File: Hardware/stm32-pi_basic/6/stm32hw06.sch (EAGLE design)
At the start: 51 parts

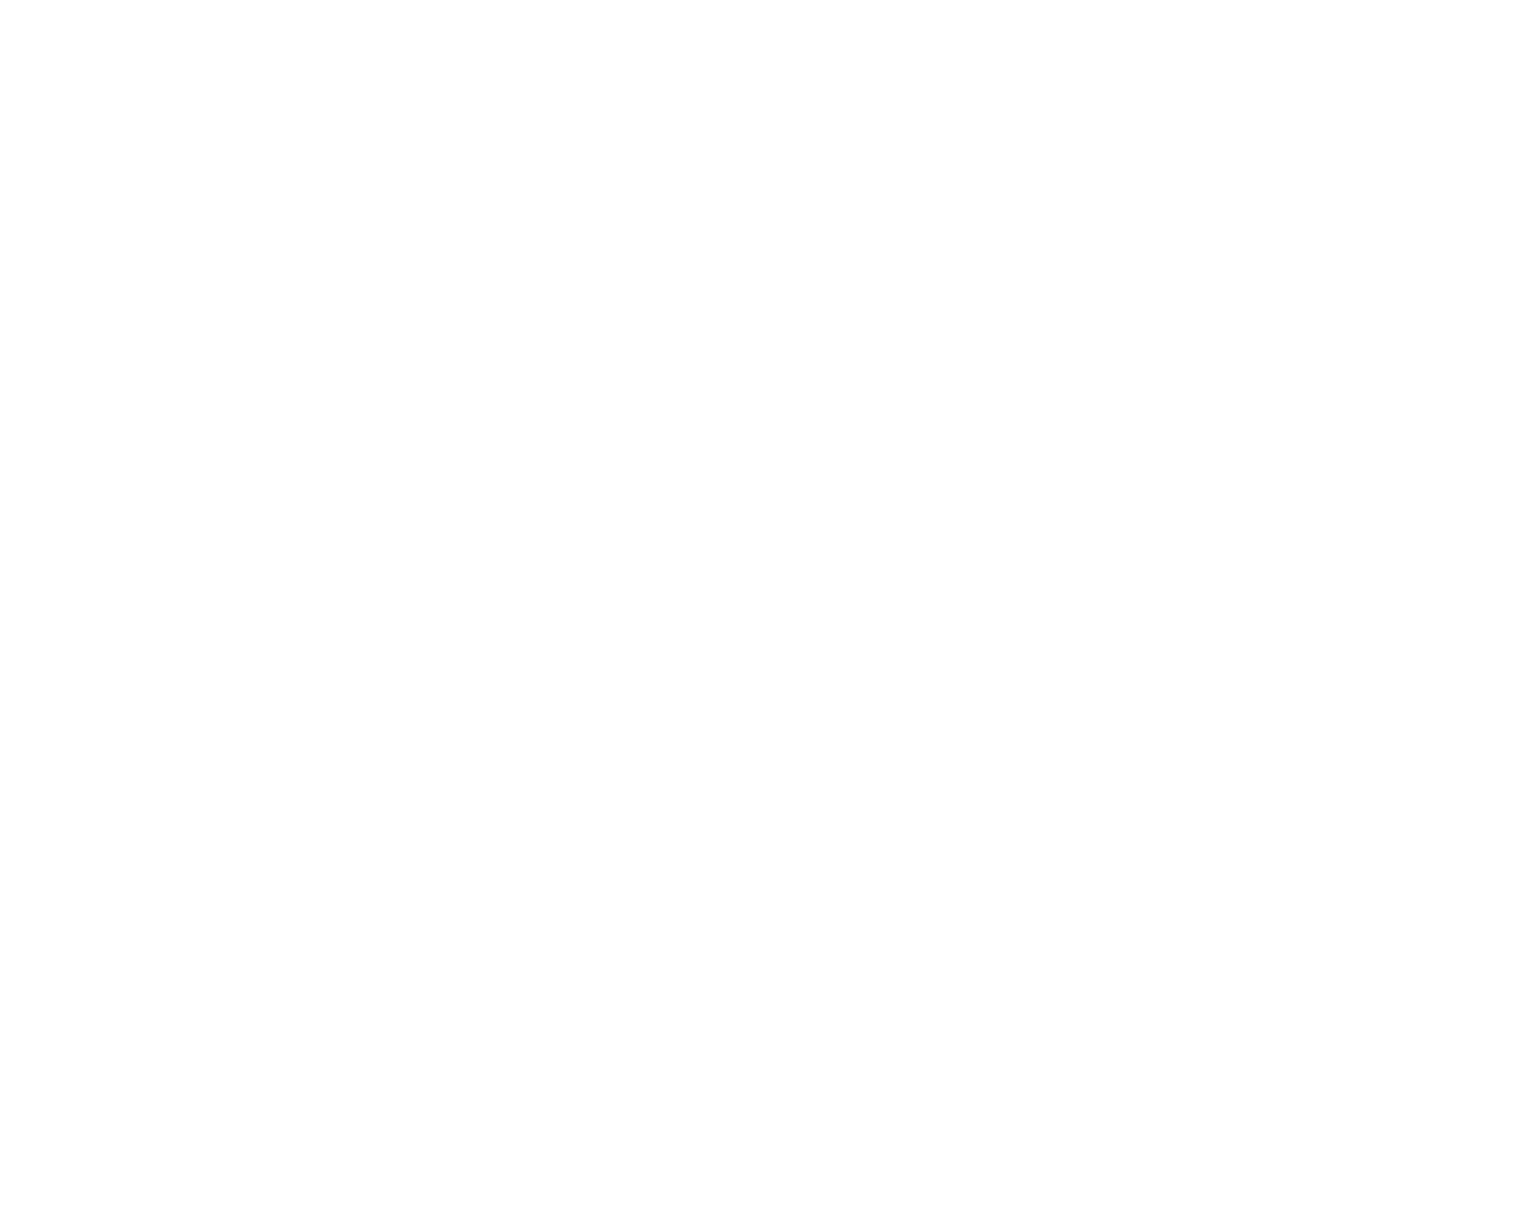
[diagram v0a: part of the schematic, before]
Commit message: deleted:    Hardware/stm32-pi_basic/6/dxfimp.scr 	modified:   Hardware/stm32-pi_basic/6/stm32hw06.brd 	modified:   Hardware/stm32-pi_basic/6/stm32hw06.sch
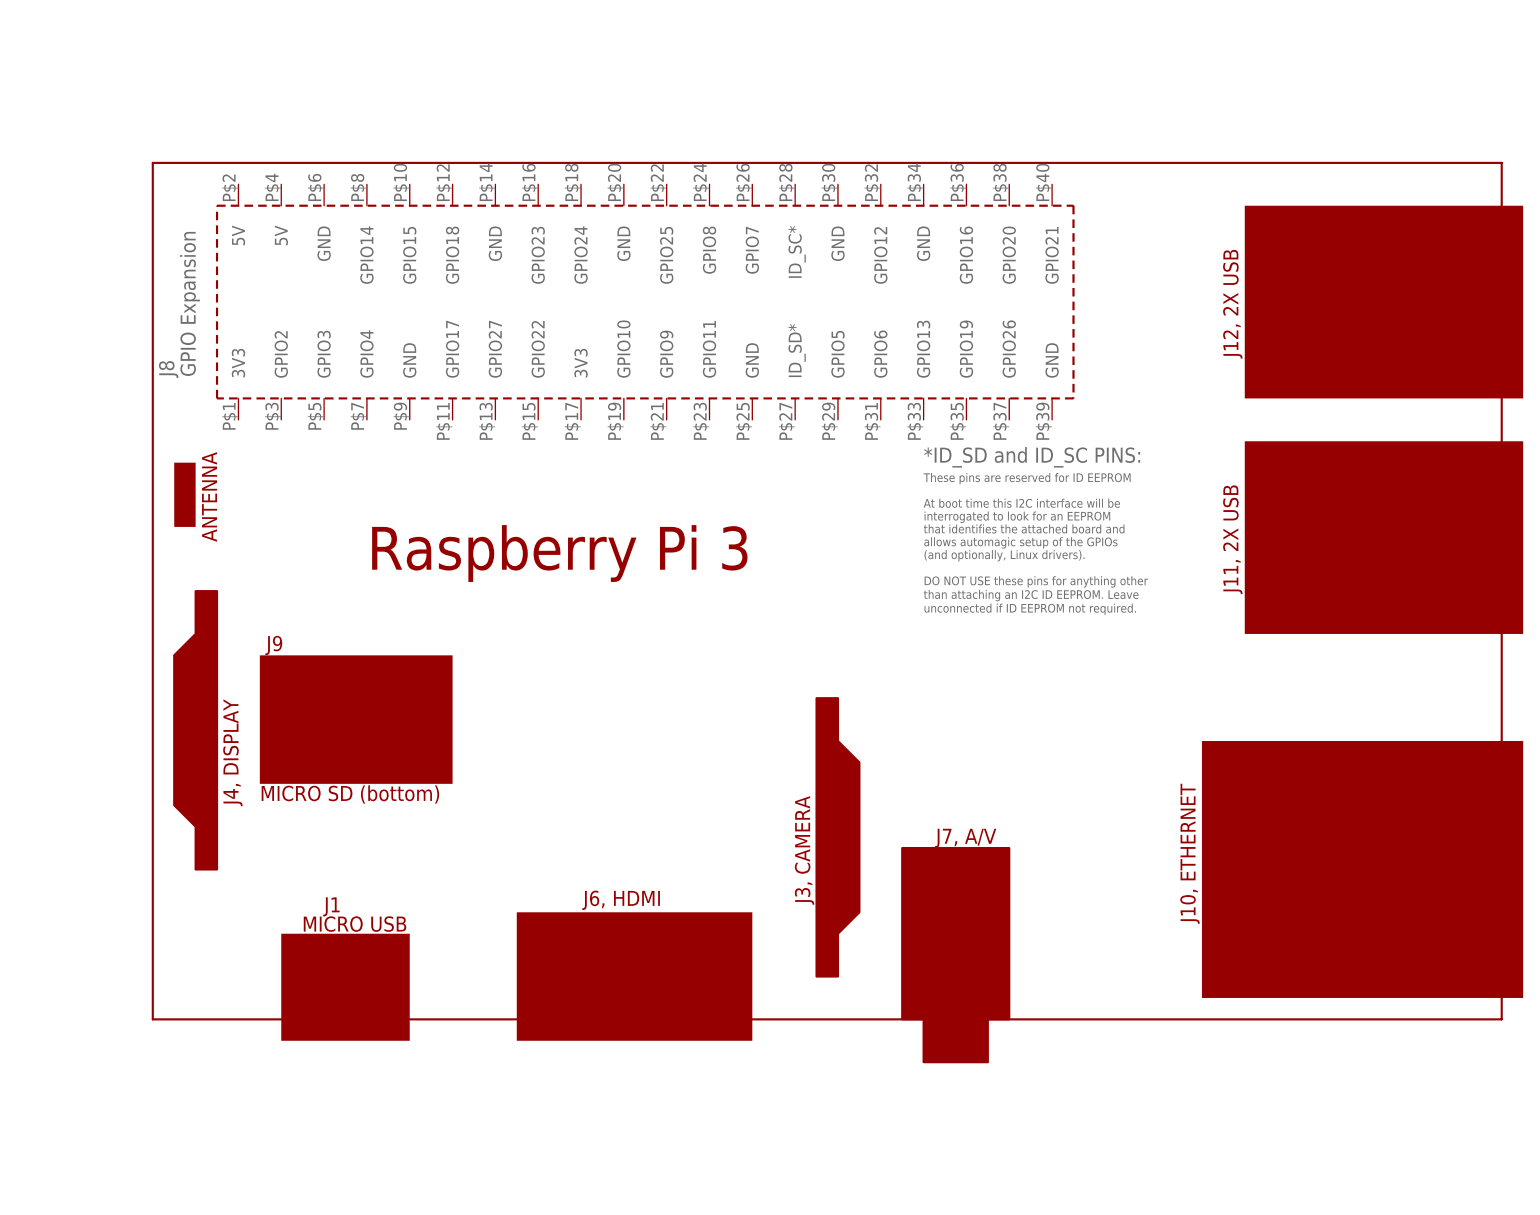
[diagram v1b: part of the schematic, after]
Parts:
- added PCB1: RPI3RPI3, e14_Rpi3_RevA+mirror-pcb:RPI3RPI3
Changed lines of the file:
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@@
 <drawing>
 <settings>
-<setting alwaysvectorfont="yes"/>
+<setting alwaysvectorfont="no"/>
 <setting keepoldvectorfont="yes"/>
 <setting verticaltext="up"/>
@@
 <part name="C2" library="resistor" deviceset="C-EU" device="C0603" value="100nF"/>
 <part name="+3V5" library="supply1" deviceset="+3V3" device=""/>
+<part name="PCB1" library="e14_Rpi3_RevA+mirror-pcb" deviceset="RPI3" device="RPI3"/>
 </parts>
 <sheets>
@@
 <attribute name="VALUE" x="-7.62" y="68.326" size="1.778" layer="96" rot="R90"/>
 </instance>
+<instance part="PCB1" gate="G$1" x="355.6" y="-203.2" smashed="yes"/>
 </instances>
 <busses>
